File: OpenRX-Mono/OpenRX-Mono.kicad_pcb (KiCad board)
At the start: 6 copper layers, 41.3 x 17.9 mm, 47 parts, among them T1 0900PC16J0042001E, U1 ESP32-C3FH4, U2 TLV75533PDQNR, U3 TS2306A 240GF MSM 9_C2976675, U4 LR1121IMLTRT, U5 OW7EL89CENUYO3YLC-32M, U7 RFX2401C, U8 SKY13414-485LF, X1 CJ17-400001010B20

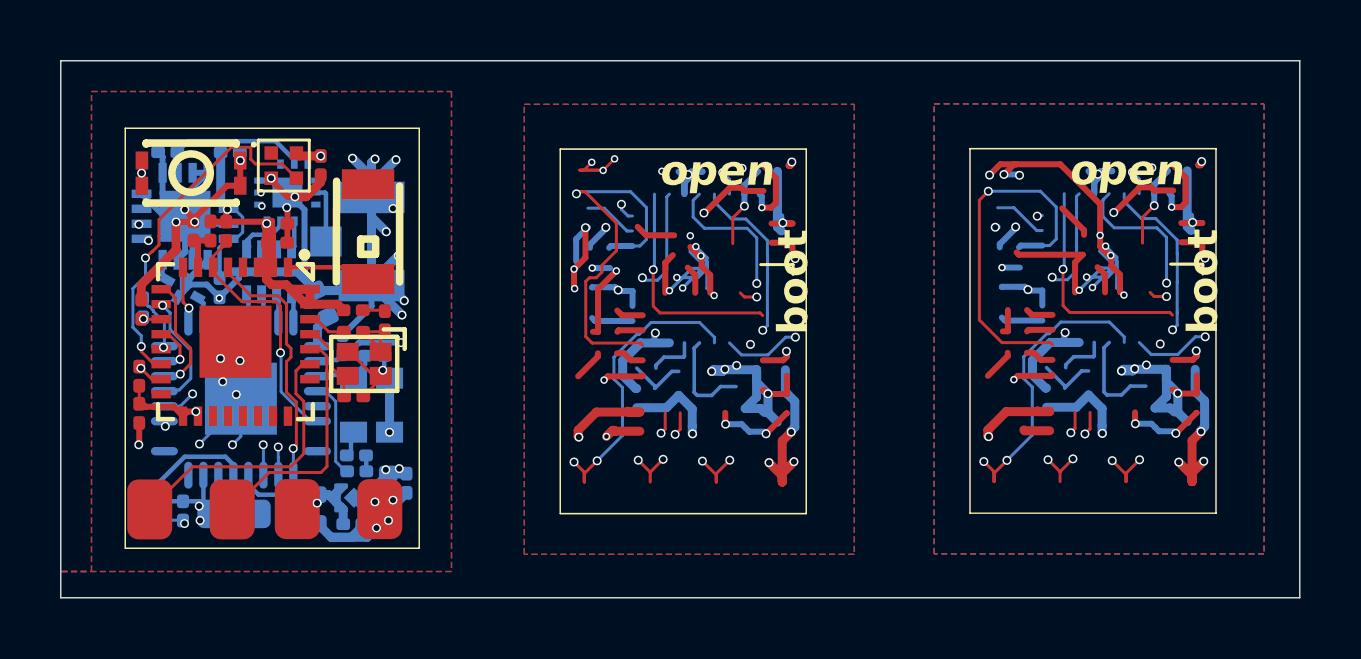
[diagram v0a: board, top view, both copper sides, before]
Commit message: initial routing for all
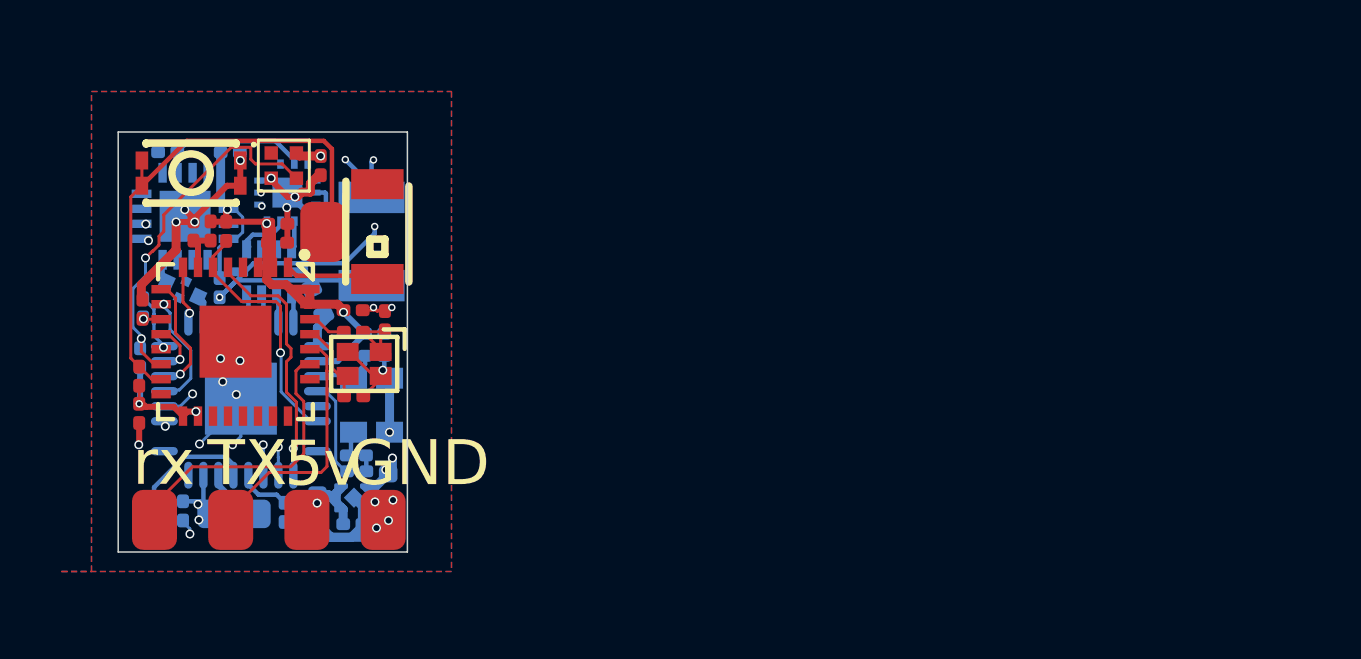
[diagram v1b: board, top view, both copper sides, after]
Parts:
- removed C10: 1uF, Capacitor_SMD:C_0201_0603Metric
- removed USB2: 2450FM07D0034, OpenRX-Shared:FILTER-SMD_4P-L1.0-W0.5-L_DEA102700LT-XXX
- added FL1: 2450FM07D0034T, OpenRX-Shared:FILTER-SMD_4P-L1.0-W0.5-L, B.Cu at (106.0, 88.6)
- added R5: 10k, Resistor_SMD:R_0201_0603Metric, B.Cu at (104.6, 90.9)
- added TP5: Boot, OpenRX-Shared:SolderPad_1.2x2.0mm, F.Cu at (110.7, 86.7)
- moved C21 1.13 mm to (112.4, 90.1), turned to 0 degrees
- moved TP3 0.48 mm to (110.2, 96.3)
- moved TP1 0.38 mm to (105.1, 96.3)
- moved TP4 0.38 mm to (112.7, 96.3)
- moved TP2 0.35 mm to (107.6, 96.3)
- moved AE1 0.31 mm to (112.5, 86.7)
- moved C20 0.17 mm to (110.5, 89.0)
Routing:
- net (no net): track 159.5 -> 0.00 mm, vias 26 -> 0
- net GND: track 157.1 -> 57.3 mm, vias 81 -> 27
- net +3V3: track 69.0 -> 30.1 mm, vias 27 -> 10
- net +5V: track 50.5 -> 15.1 mm, vias 10 -> 2
- net Net-(U1-U0RXD): track 30.7 -> 9.33 mm, vias 6 -> 0
- net Net-(U1-U0TXD): track 27.8 -> 8.09 mm, vias 4 -> 0
- net /ESP32-C3 + LR1121 Mono/BUTTON: track 8.89 -> 18.2 mm, vias 2 -> 0
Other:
- board size 41.3 x 17.9 mm -> 9.6 x 14 mm
- board text added: "rx"
- board text removed: "RX"
- board text removed: "boot"
- board text removed: "open"

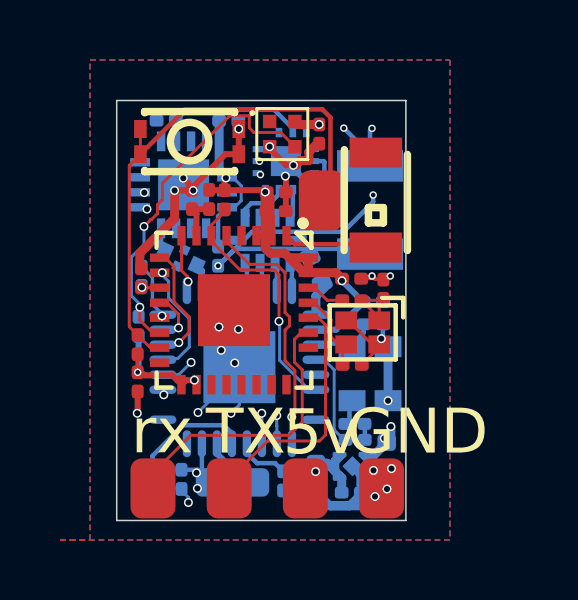
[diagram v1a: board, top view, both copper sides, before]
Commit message: final route
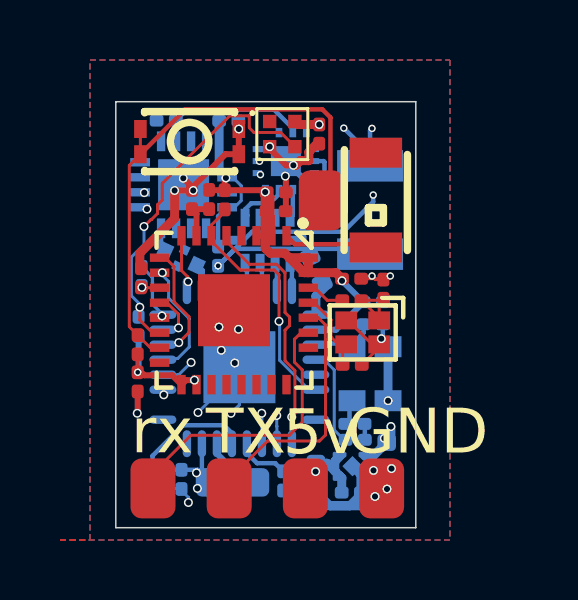
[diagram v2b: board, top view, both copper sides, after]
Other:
- board size 9.6 x 14 mm -> 10 x 14.2 mm
